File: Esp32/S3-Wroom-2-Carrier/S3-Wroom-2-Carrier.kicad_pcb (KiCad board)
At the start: 6 copper layers, 29 x 39 mm, 14 parts, among them J1 DF9-21S-1V32, J2 DF9-21S-1V32, J3 USB_C_Receptacle_USB2.0_16P, U2 ADM7171ACPZ-3.0-R7

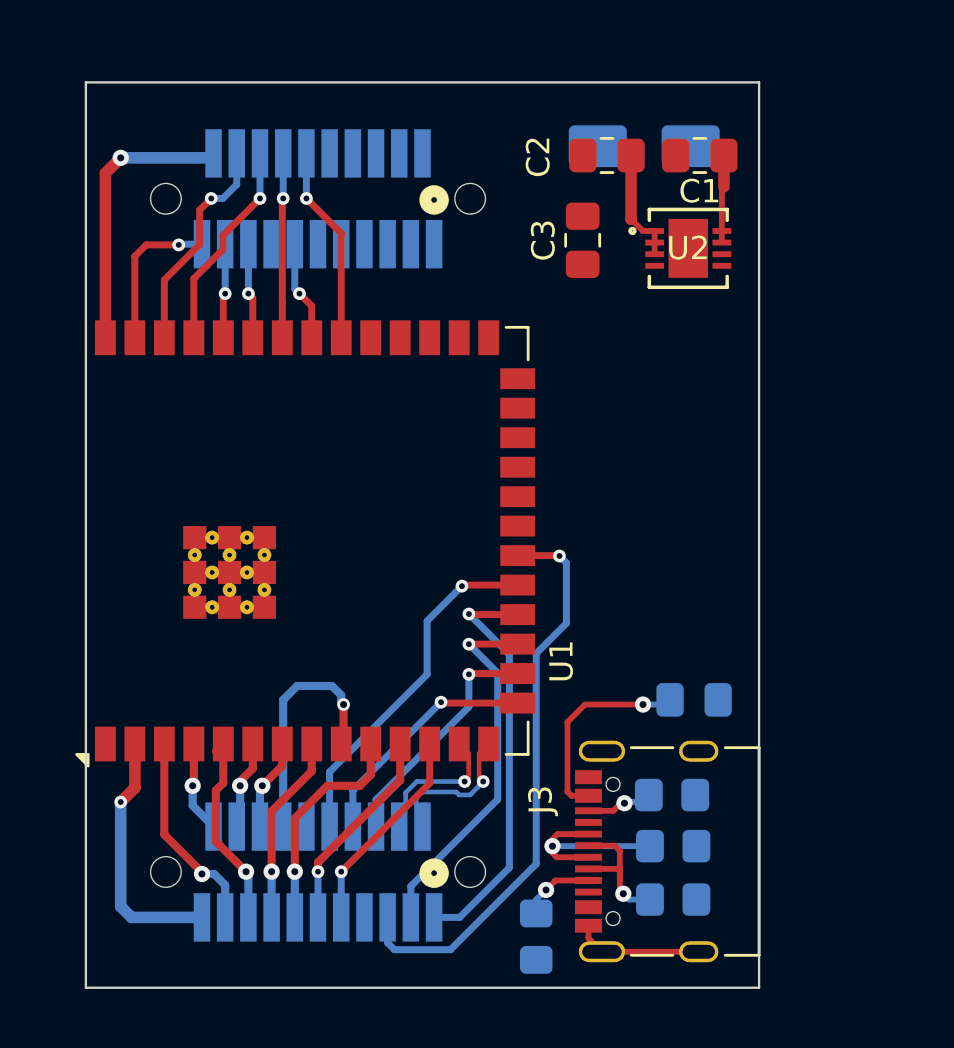
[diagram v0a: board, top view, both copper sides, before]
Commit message: Routing
Routing finished needs to be verify
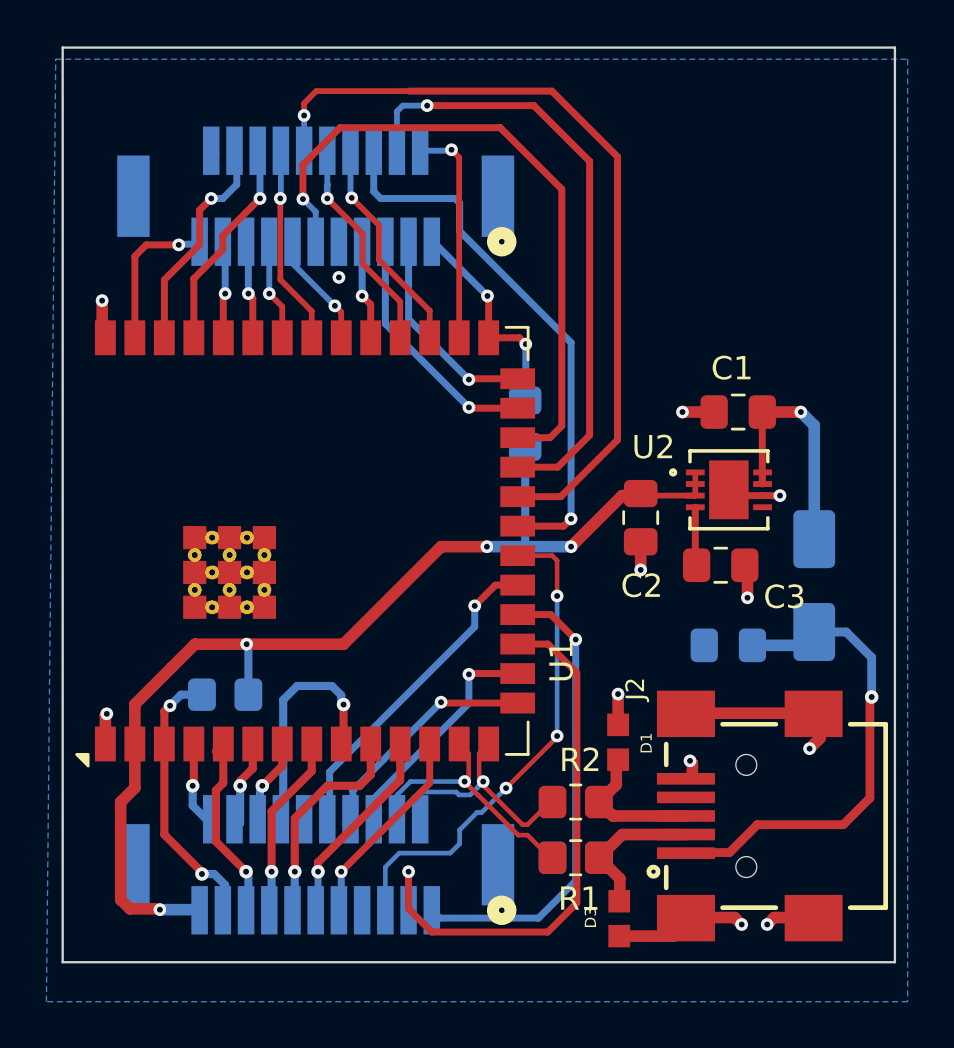
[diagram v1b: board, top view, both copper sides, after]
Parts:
- removed J1: DF9-21S-1V32, Library:CON9_1X21_DZL_DF9_HIR
- removed J3: USB_C_Receptacle_USB2.0_16P, Connector_USB:USB_C_Receptacle_Palconn_UTC16-G
- removed R4: 5K1, Resistor_SMD:R_0805_2012Metric_Pad1.20x1.40mm_HandSolder
- added D1: ~, User_Footprint:DIOC1608X36N, F.Cu at (159.4, 108.4)
- added D3: ~, User_Footprint:DIOC1608X36N, F.Cu at (159.5, 116.0)
- added J4: DF9B-21S-1V69, User_Footprint:CONN_DF9B-21S-1V_21P_HIR, B.Cu at (146.4, 113.8)
- added J5: DF9B-21S-1V69, User_Footprint:CONN_DF9B-21S-1V_21P_HIR, B.Cu at (146.4, 85.0)
- added R5: 10K, Resistor_SMD:R_0805_2012Metric_Pad1.20x1.40mm_HandSolder, B.Cu at (142.5, 106.4)
- added R6: 10K, Resistor_SMD:R_0805_2012Metric_Pad1.20x1.40mm_HandSolder, B.Cu at (155.4, 94.7)
- J2: value DF9-21S-1V32 -> 65100516121; footprint Library:CON9_1X21_DZL_DF9_HIR -> User_Footprint:Usb_B_mini_Wurth_65100516121; moved to F.Cu
- R1, R2: moved to F.Cu
- moved D2 20.3 mm to (167.9, 101.7), turned to -90 degrees
- moved J2 19.9 mm to (166.2, 111.6), turned to 90 degrees
- moved C2 15.7 mm to (160.4, 98.8), turned to -90 degrees
- moved C3 15.2 mm to (163.8, 100.8), turned to 0 degrees
- moved C1 11.2 mm to (164.6, 94.2)
- moved U2 10.5 mm to (164.2, 97.6)
- moved R2 4.61 mm to (157.6, 111.0), turned to 0 degrees
- moved R1 4.57 mm to (157.6, 113.4), turned to 0 degrees
- moved R3 3.80 mm to (157.6, 113.4), turned to 0 degrees
- moved C4 2.77 mm to (164.2, 104.2), turned to 180 degrees
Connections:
- C4 pad 1: Net-(D2-A) -> /Project Architecture/Power/VBUS
- D2 pad 2: Net-(D2-A) -> /Project Architecture/Power/VBUS
- J2 pad 1: /Project Architecture/Break Out Connection/GPIO10 -> /Project Architecture/Power/VBUS
- J2 pad 2: /Project Architecture/Break Out Connection/USB_D+ -> Net-(J2-D-)
- J2 pad 3: /Project Architecture/Break Out Connection/GPIO9 -> Net-(J2-D+)
- J2 pad 4: /Project Architecture/Break Out Connection/USB_D- -> unconnected-(J2-ID-Pad4)
- J2 pad 5: /Project Architecture/Break Out Connection/GPIO12 -> GND
- R1 pad 2: Net-(J3-D--PadA7) -> Net-(J2-D-)
- R2 pad 2: Net-(J3-D+-PadA6) -> Net-(J2-D+)
- U1 pad 28: unconnected-(U1C-NC-Pad28) -> /Project Architecture/Break Out Connection/GPIO35
- U1 pad 29: unconnected-(U1C-NC-Pad29) -> /Project Architecture/Break Out Connection/GPIO36
- U1 pad 30: unconnected-(U1C-NC-Pad30) -> /Project Architecture/Break Out Connection/GPIO37
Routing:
- net /Project Architecture/Break Out Connection/GPIO14: track 0.00 -> 34.4 mm, vias 0 -> 1
- net +3V3: track 16.1 -> 47.7 mm, vias 1 -> 4
- net /Project Architecture/Break Out Connection/GPIO47: track 0.00 -> 28.8 mm, vias 0 -> 1
- net /Project Architecture/Break Out Connection/GPIO21: track 0.00 -> 26.6 mm, vias 0 -> 1
- net /Project Architecture/Break Out Connection/GPIO13: track 0.00 -> 23.7 mm, vias 0 -> 1
- net GND: track 17.6 -> 38.3 mm, vias 1 -> 12
- net /Project Architecture/Power/VBUS: track 0.00 -> 20.5 mm, vias 0 -> 1
- net /Project Architecture/Break Out Connection/GPIO48: track 0.00 -> 10.7 mm, vias 0 -> 1
- net /Project Architecture/Break Out Connection/GPIO37: track 0.00 -> 9.97 mm, vias 0 -> 1
- net /Project Architecture/Break Out Connection/GPIO35: track 0.00 -> 9.60 mm, vias 0 -> 1
- net /Project Architecture/Break Out Connection/GPIO36: track 0.00 -> 9.47 mm, vias 0 -> 1
- net /Project Architecture/Break Out Connection/GPIO0: track 0.00 -> 9.34 mm, vias 0 -> 2
- net /Project Architecture/Break Out Connection/GPIO45: track 0.00 -> 9.13 mm, vias 0 -> 1
- net Net-(D2-A): track 8.79 -> 0.00 mm, vias 1 -> 0
- net /Project Architecture/Break Out Connection/GPIO9: track 15.9 -> 24.4 mm
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- added copper zone on B.Cu, net GND
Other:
- board size 29 x 39 mm -> 35.8 x 39.4 mm
- copper layers 6 -> 2
